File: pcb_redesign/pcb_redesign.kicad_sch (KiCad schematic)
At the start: 7 parts, among them U1 ESP32-S3-WROOM-1

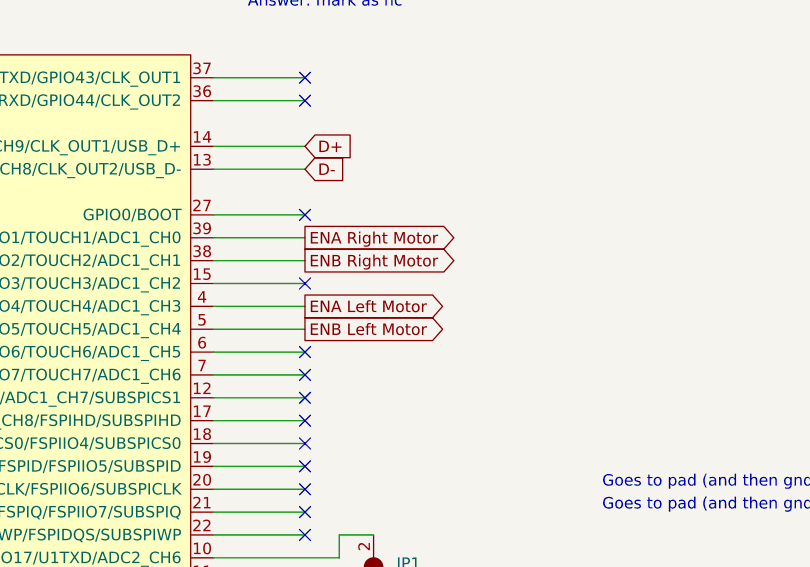
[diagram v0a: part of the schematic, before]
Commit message: switching to laptop
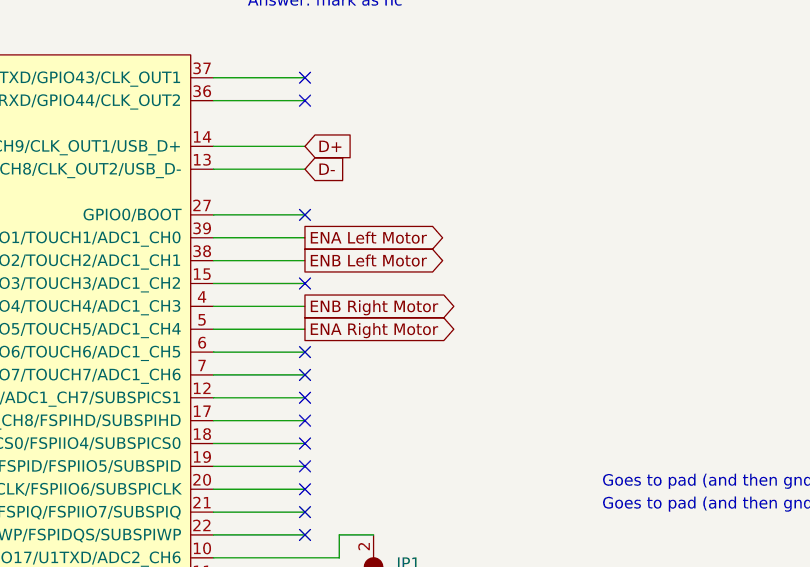
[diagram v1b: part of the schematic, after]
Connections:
- net ENA Left Motor: now also U1.39 (GPIO1/TOUCH1/ADC1_CH0); no longer U1.4 (GPIO4/TOUCH4/ADC1_CH3)
- net ENA Right Motor: now also U1.5 (GPIO5/TOUCH5/ADC1_CH4); no longer U1.39 (GPIO1/TOUCH1/ADC1_CH0)
- net ENB Left Motor: now also U1.38 (GPIO2/TOUCH2/ADC1_CH1); no longer U1.5 (GPIO5/TOUCH5/ADC1_CH4)
- net ENB Right Motor: now also U1.4 (GPIO4/TOUCH4/ADC1_CH3); no longer U1.38 (GPIO2/TOUCH2/ADC1_CH1)
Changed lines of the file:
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@@
     )
   )
-  (global_label "ENB Left Motor" (shape output) (at 199.39 86.36 0) (fields_autoplaced)
+  (global_label "ENA Right Motor" (shape output) (at 199.39 86.36 0) (fields_autoplaced)
     (effects (font (size 1.27 1.27)) (justify left))
-    (property "Intersheetrefs" "${INTERSHEET_REFS}" (at 216.8099 86.36 0)
+    (property "Intersheetrefs" "${INTERSHEET_REFS}" (at 217.9589 86.36 0)
       (effects (font (size 1.27 1.27)) (justify left) hide)
     )
   )
-  (global_label "ENA Left Motor" (shape output) (at 199.39 83.82 0) (fields_autoplaced)
+  (global_label "ENA Left Motor" (shape output) (at 199.39 76.2 0) (fields_autoplaced)
     (effects (font (size 1.27 1.27)) (justify left))
-    (property "Intersheetrefs" "${INTERSHEET_REFS}" (at 216.6285 83.82 0)
+    (property "Intersheetrefs" "${INTERSHEET_REFS}" (at 216.6285 76.2 0)
       (effects (font (size 1.27 1.27)) (justify left) hide)
     )
@@
     )
   )
+  (global_label "ENB Right Motor" (shape output) (at 199.39 83.82 0) (fields_autoplaced)
+    (effects (font (size 1.27 1.27)) (justify left))
+    (property "Intersheetrefs" "${INTERSHEET_REFS}" (at 218.1403 83.82 0)
+      (effects (font (size 1.27 1.27)) (justify left) hide)
+    )
+  )
   (global_label "D-" (shape input) (at 199.39 68.58 0) (fields_autoplaced)
     (effects (font (size 1.27 1.27)) (justify left))
     (property "Intersheetrefs" "${INTERSHEET_REFS}" (at 205.1382 68.58 0)
-      (effects (font (size 1.27 1.27)) (justify left) hide)
-    )
-  )
-  (global_label "ENA Right Motor" (shape output) (at 199.39 76.2 0) (fields_autoplaced)
-    (effects (font (size 1.27 1.27)) (justify left))
-    (property "Intersheetrefs" "${INTERSHEET_REFS}" (at 217.9589 76.2 0)
-      (effects (font (size 1.27 1.27)) (justify left) hide)
-    )
-  )
-  (global_label "ENB Right Motor" (shape output) (at 199.39 78.74 0) (fields_autoplaced)
-    (effects (font (size 1.27 1.27)) (justify left))
-    (property "Intersheetrefs" "${INTERSHEET_REFS}" (at 218.1403 78.74 0)
       (effects (font (size 1.27 1.27)) (justify left) hide)
     )
@@
     )
   )
+  (global_label "ENB Left Motor" (shape output) (at 199.39 78.74 0) (fields_autoplaced)
+    (effects (font (size 1.27 1.27)) (justify left))
+    (property "Intersheetrefs" "${INTERSHEET_REFS}" (at 216.8099 78.74 0)
+      (effects (font (size 1.27 1.27)) (justify left) hide)
+    )
+  )
